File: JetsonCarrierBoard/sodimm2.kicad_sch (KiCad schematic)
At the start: 1 part

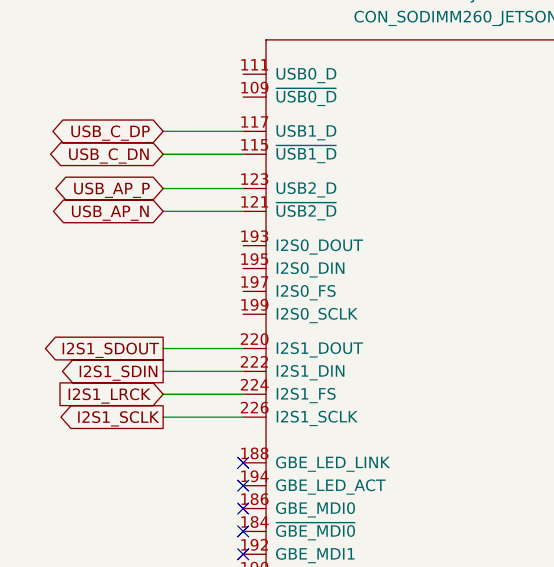
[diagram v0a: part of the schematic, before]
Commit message: Small changes
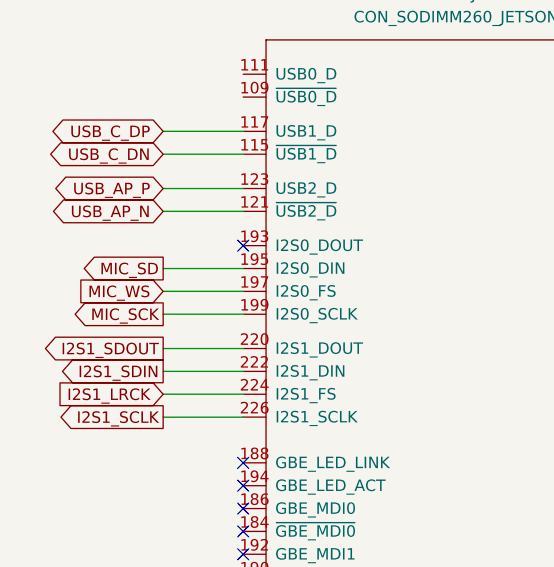
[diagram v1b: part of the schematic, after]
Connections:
- net MIC_SD: now reaches J?.195 (I2S0_DIN)
- net MIC_WS: now reaches J?.197 (I2S0_FS)
- net MIC_SCK: now reaches J?.199 (I2S0_SCLK)
- no-connect marks 16 -> 17
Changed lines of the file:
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@@
   (no_connect (at 116.84 78.74))
   (no_connect (at 116.84 81.28))
+  (no_connect (at 116.84 46.99))
   (wire (pts (xy 107.95 63.5) (xy 116.84 63.5))
+    (stroke (width 0) (type default) (color 0 0 0 0))
+  )
+  (wire (pts (xy 107.95 52.07) (xy 116.84 52.07))
     (stroke (width 0) (type default) (color 0 0 0 0))
   )
@@
   )
   (wire (pts (xy 107.95 34.29) (xy 116.84 34.29))
+    (stroke (width 0) (type default) (color 0 0 0 0))
+  )
+  (wire (pts (xy 107.95 49.53) (xy 116.84 49.53))
     (stroke (width 0) (type default) (color 0 0 0 0))
   )
@@
   )
   (wire (pts (xy 107.95 40.64) (xy 116.84 40.64))
+    (stroke (width 0) (type default) (color 0 0 0 0))
+  )
+  (wire (pts (xy 107.95 54.61) (xy 116.84 54.61))
     (stroke (width 0) (type default) (color 0 0 0 0))
   )
@@
     )
   )
+  (global_label "MIC_SCK" (shape output) (at 107.95 54.61 180) (fields_autoplaced)
+    (effects (font (size 1.27 1.27)) (justify right))
+    (property "Intersheet References" "${INTERSHEET_REFS}" (id 0) (at 97.4936 54.5306 0)
+      (effects (font (size 1.27 1.27)) (justify right) hide)
+    )
+  )
   (global_label "I2S1_SDIN" (shape output) (at 107.95 60.96 180) (fields_autoplaced)
     (effects (font (size 1.27 1.27)) (justify right))
@@
       (effects (font (size 1.27 1.27)) (justify right) hide)
     )
+  )
+  (global_label "MIC_WS" (shape input) (at 107.95 52.07 180) (fields_autoplaced)
+    (effects (font (size 1.27 1.27)) (justify right))
+    (property "Intersheet References" "${INTERSHEET_REFS}" (id 0) (at 98.5821 52.1494 0)
+      (effects (font (size 1.27 1.27)) (justify right) hide)
+    )
+  )
+  (global_label "MIC_SD" (shape output) (at 107.95 49.53 180) (fields_autoplaced)
+    (effects (font (size 1.27 1.27)) (justify right))
+    (property "Intersheet References" "${INTERSHEET_REFS}" (id 0) (at 98.7636 49.4506 0)
+      (effects (font (size 1.27 1.27)) (justify right) hide)
+    )
